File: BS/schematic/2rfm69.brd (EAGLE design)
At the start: 100 x 50 mm, 17 parts, among them IC1 Atmega328P-PU, IC2 FT232R, Q1 16MHz, U1 RFM69, X1 PN61729-S

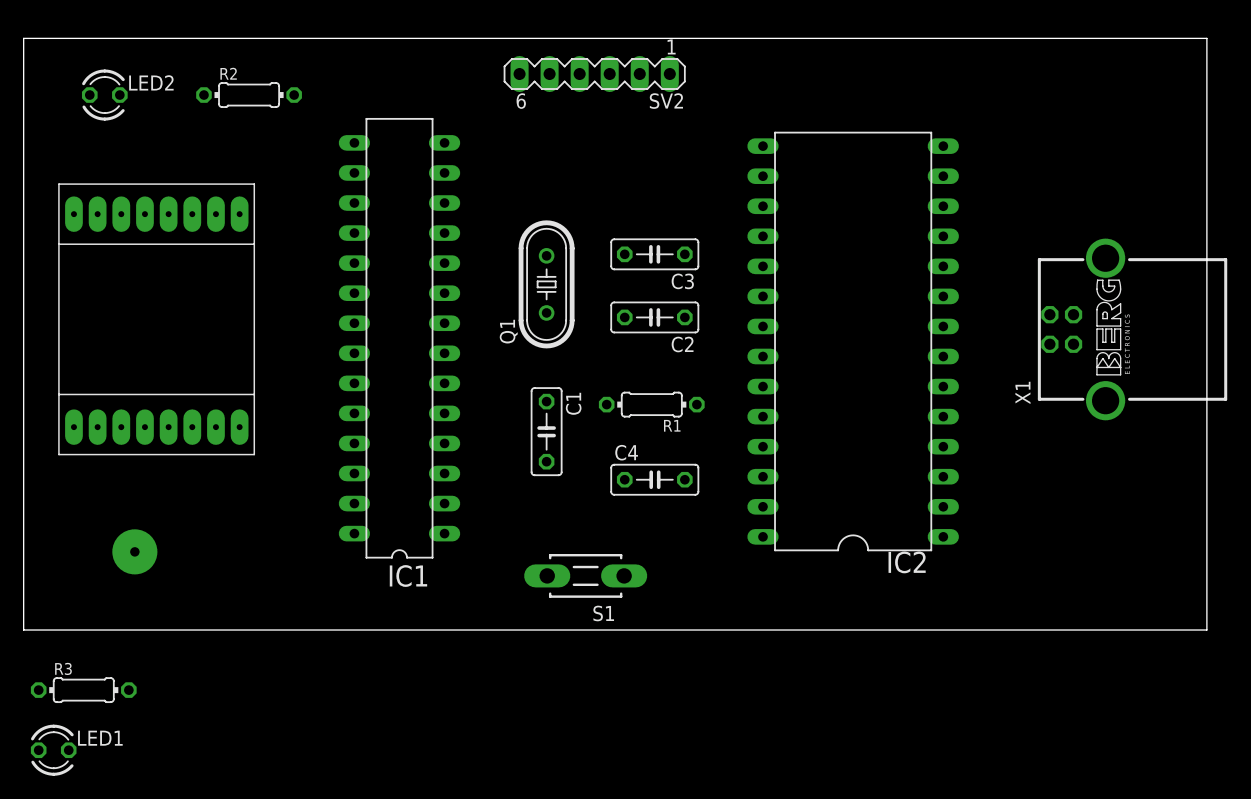
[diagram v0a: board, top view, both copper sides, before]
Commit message: Test schematic BS
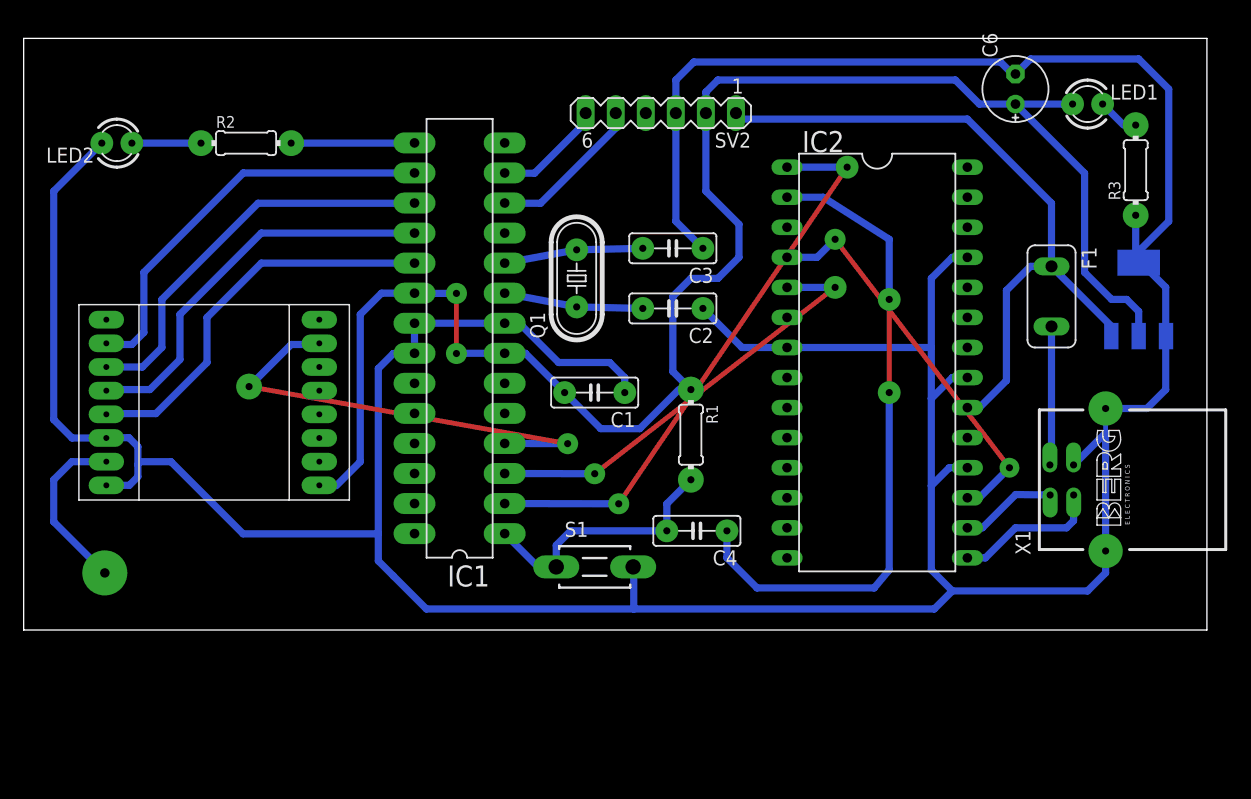
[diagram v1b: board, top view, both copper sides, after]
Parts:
- added C6: 10uF, rcl:E2,5-6E
- added F1: 500mA, fuse:TE5
- added U$1: LM1117, 1117:SOT223
- moved LED1 103.0 mm to (89.9, 44.5)
- moved R3 99.2 mm to (94.0, 38.9), turned to 90 degrees
- moved X1 12.7 mm to (91.4, 12.7)
- moved U1 8.42 mm to (16.1, 19.9), turned to 270 degrees
- moved SV2 6.49 mm to (53.8, 43.7)
- moved C4 5.59 mm to (56.9, 8.38), turned to 180 degrees
- moved C1 5.24 mm to (48.3, 20.1), turned to 180 degrees
- moved IC1 5.08 mm to (36.8, 24.7)
- moved LED2 4.19 mm to (7.87, 41.1), turned to 180 degrees
- moved R1 4.17 mm to (56.4, 16.5), turned to 270 degrees
- moved R2 4.07 mm to (18.8, 41.1)
- moved U$2 3.10 mm to (6.86, 4.83)
- moved IC2 2.70 mm to (72.1, 22.6), turned to 270 degrees
- moved Q1 2.59 mm to (46.7, 29.7)
- moved C2 1.70 mm to (54.9, 27.2)
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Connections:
- removed net VCCIO: IC2.VCCIO
- new net 3V3_FTDI: IC2.3V3OUT, IC2.VCCIO
- new net N$5: LED1.K, R3.2
- new net N$8: F1.2, X1.1
- net +3V3: now also C6.+, LED1.A, SV2.2, U$1.VOUT
- net +5V: now also F1.1, SV2.1, U$1.VIN; no longer X1.1
- net D6: now also SV2.5
- net D7: now also SV2.6
- net GND: now also C6.-, R3.1, SV2.3, U$1.GND, U$1.GND1
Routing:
- net GND: track 0.00 -> 359.0 mm
- net +3V3: track 0.00 -> 142.1 mm, vias 0 -> 2
- net +5V: track 0.00 -> 59.7 mm
- net N$3: track 0.00 -> 55.4 mm, vias 0 -> 2
- net D0_RX: track 0.00 -> 49.1 mm, vias 0 -> 2
- net D2_INT: track 0.00 -> 40.1 mm, vias 0 -> 2
- net D1_TX: track 0.00 -> 37.4 mm, vias 0 -> 2
- net D10_SS1: track 0.00 -> 35.1 mm
- net D11_MOSI: track 0.00 -> 34.2 mm
- net D12_MISO: track 0.00 -> 33.8 mm
- net 3V3_FTDI: track 0.00 -> 33.6 mm, vias 0 -> 2
- net D13_SCK: track 0.00 -> 33.6 mm
- net RST: track 0.00 -> 22.4 mm
- net N$4: track 0.00 -> 14.7 mm
- net D6: track 0.00 -> 13.3 mm
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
